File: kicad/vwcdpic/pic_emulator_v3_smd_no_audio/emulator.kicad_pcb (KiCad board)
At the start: 2 copper layers, 48.1 x 36.8 mm, 48 parts, among them P1 CONN_01X05, P2 CONN_01X02, U1 PIC12F629, U2 78L05

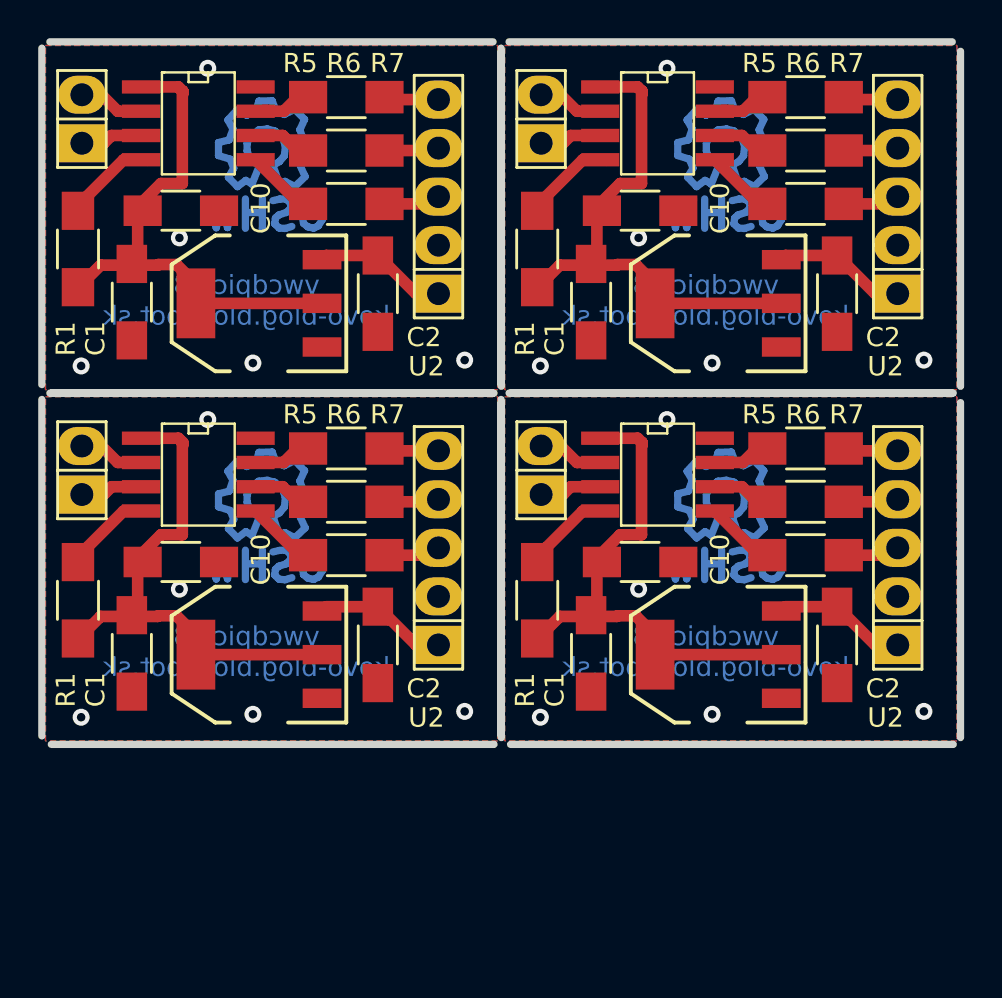
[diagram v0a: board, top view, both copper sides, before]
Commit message: ..
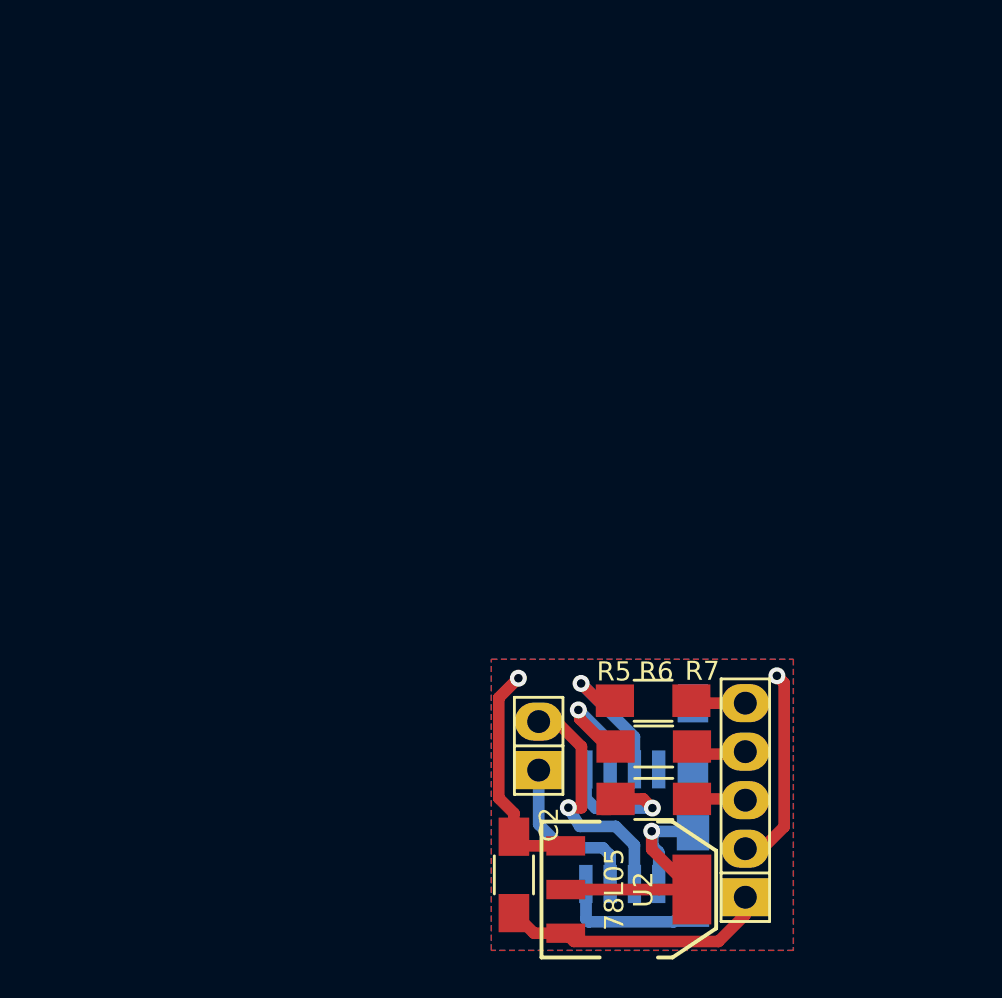
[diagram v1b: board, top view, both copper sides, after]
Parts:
- removed C1 (x4): 100n, Capacitors_SMD:C_1206_HandSoldering
- removed the C10 at (120.8, 106.5)
- removed the C10 at (120.8, 88.1)
- removed the C10 at (144.9, 88.1)
- removed the C10 at (144.9, 106.5)
- removed the C2 at (131.1, 110.8)
- removed the C2 at (131.1, 92.4)
- removed the C2 at (155.2, 92.4)
- removed the C2 at (155.2, 110.8)
- removed the P1 at (134.3, 105.7)
- removed the P1 at (134.3, 87.4)
- removed the P1 at (158.3, 87.4)
- removed the P1 at (158.3, 105.7)
- removed the P2 at (115.6, 101.7)
- removed the P2 at (115.6, 83.3)
- removed the P2 at (139.7, 83.3)
- removed the P2 at (139.7, 101.7)
- removed the R1 at (115.4, 108.5)
- removed the R1 at (115.4, 90.1)
- removed the R1 at (139.5, 90.1)
- removed the R1 at (139.5, 108.5)
- removed the R5 at (129.5, 100.5)
- removed the R5 at (129.5, 82.1)
- removed the R5 at (153.5, 82.1)
- removed the R5 at (153.5, 100.5)
- removed the R6 at (129.5, 103.3)
- removed the R6 at (129.5, 84.9)
- removed the R6 at (153.5, 84.9)
- removed the R6 at (153.5, 103.3)
- removed the R7 at (129.5, 106.1)
- removed the R7 at (129.5, 87.7)
- removed the R7 at (153.5, 87.7)
- removed the R7 at (153.5, 106.1)
- removed SYM (x4): Symbol_OSHW-Logo_CopperTop_07Jul2012, Symbols:Symbol_OSHW-Logo_CopperTop
- removed the U1 at (121.7, 101.9)
- removed the U1 at (121.7, 83.5)
- removed the U1 at (145.8, 83.5)
- removed the U1 at (145.8, 101.9)
- removed the U2 at (124.9, 111.3)
- removed the U2 at (124.9, 92.9)
- removed the U2 at (148.9, 92.9)
- removed the U2 at (148.9, 111.3)
- added C10: 100n, Capacitors_SMD:C_1206_HandSoldering, B.Cu at (147.6, 115.9)
- added C2: 100n, Capacitors_SMD:C_1206_HandSoldering, F.Cu at (138.3, 122.9)
- added P1: CONN_01X05, Pin_Headers:Pin_Header_Straight_1x05, F.Cu at (150.4, 118.9)
- added P2: CONN_01X02, Pin_Headers:Pin_Header_Straight_1x02, F.Cu at (139.5, 116.1)
- added R1: 10k, Resistors_SMD:R_1206_HandSoldering, B.Cu at (147.6, 122.6)
- added R5: 3k3, Resistors_SMD:R_1206_HandSoldering, F.Cu at (145.5, 113.7)
- added R6: 3k3, Resistors_SMD:R_1206_HandSoldering, F.Cu at (145.6, 116.1)
- added R7: 3k3, Resistors_SMD:R_1206_HandSoldering, F.Cu at (145.6, 118.9)
- added U1: PIC12F629, my_modules:SOIC-8-W_long_pads, B.Cu at (143.9, 120.3)
- added U2: 78L05, my_modules:SOT-223-REGULATOR, F.Cu at (144.3, 123.6)
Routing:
- net +5V: track 113.8 -> 18.3 mm, vias 0 -> 1
- net GND: track 0.00 -> 22.5 mm, vias 0 -> 2
- net POWER_CTL: track 28.1 -> 14.9 mm
- net Net-(R1-Pad1): track 19.5 -> 7.81 mm
- net DataOut: track 14.7 -> 4.04 mm
- net DataIn: track 13.0 -> 3.24 mm
- net CLK: track 12.4 -> 3.09 mm
- net Net-(R7-Pad1): track 16.5 -> 8.19 mm, vias 0 -> 1
- net Net-(R6-Pad1): track 12.7 -> 7.00 mm, vias 0 -> 1
- net Net-(P2-Pad1): track 13.1 -> 8.76 mm
- net Net-(R5-Pad1): track 12.2 -> 8.34 mm, vias 0 -> 1
- net Net-(P2-Pad2): track 16.3 -> 13.1 mm, vias 0 -> 1
- net (no net): vias 20 -> 0
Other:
- board outline removed
- net class Default: clearance 0.254 -> 0.1
- net class GND: clearance 0.254 -> 0.1
- rule trace_clearance: 0.254 -> 0.1
- board text removed: "vwcdpic v3 kovo-blog.blogspot.sk"
